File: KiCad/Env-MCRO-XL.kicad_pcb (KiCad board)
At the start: 2 copper layers, 47 parts, among them SW1 RotaryEncoder_Switch, SW2 RotaryEncoder_Switch, SW3 RotaryEncoder_Switch, U1 Pico

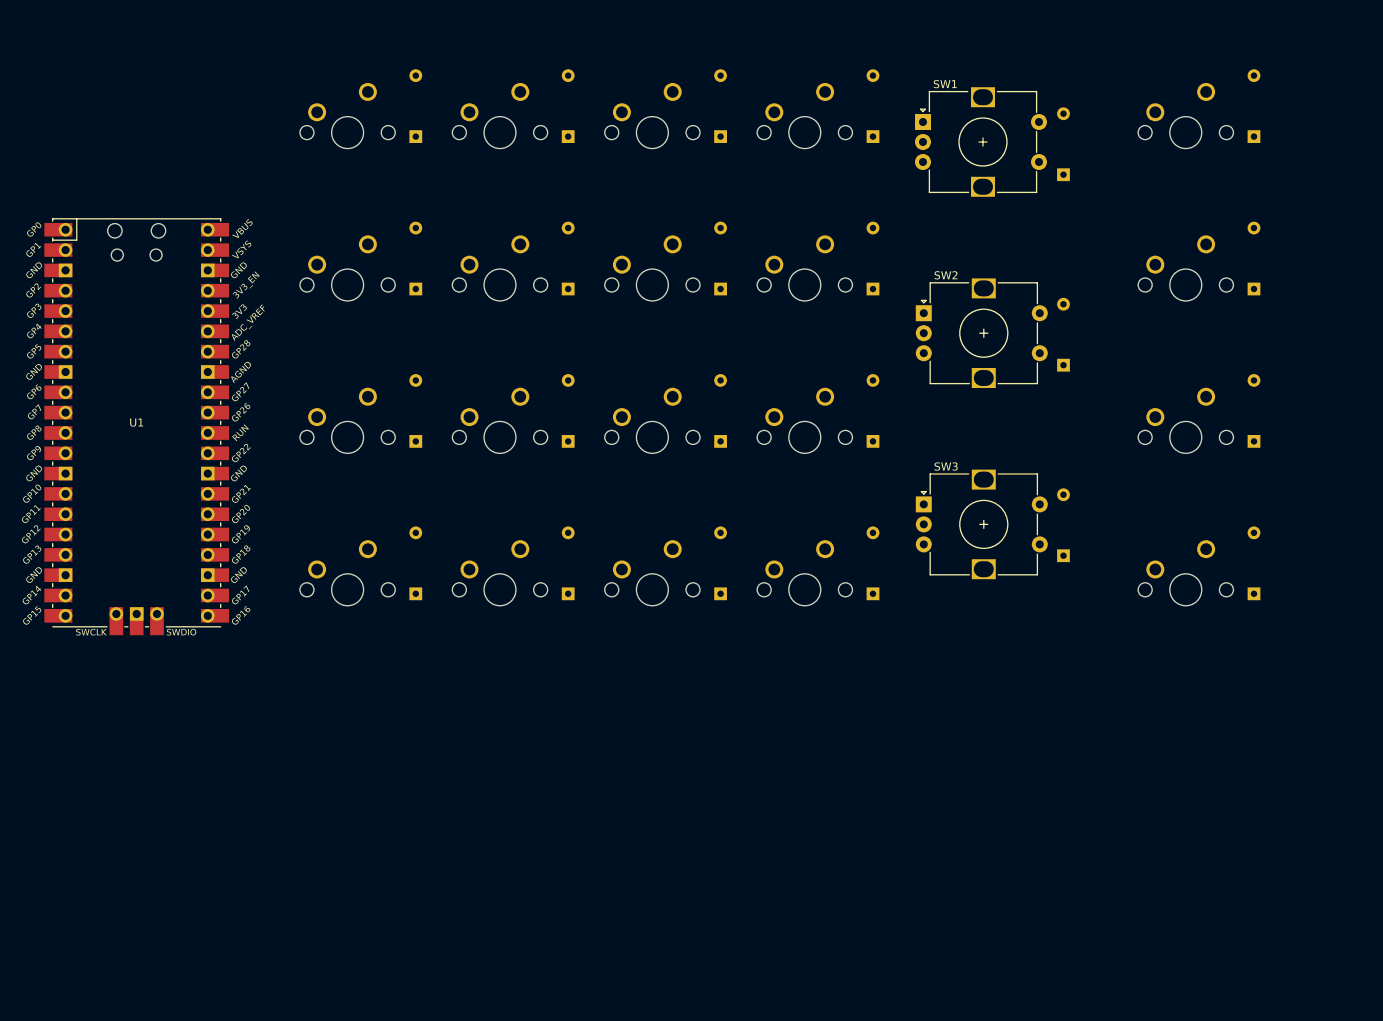
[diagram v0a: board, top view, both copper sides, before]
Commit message: initial commit + 2
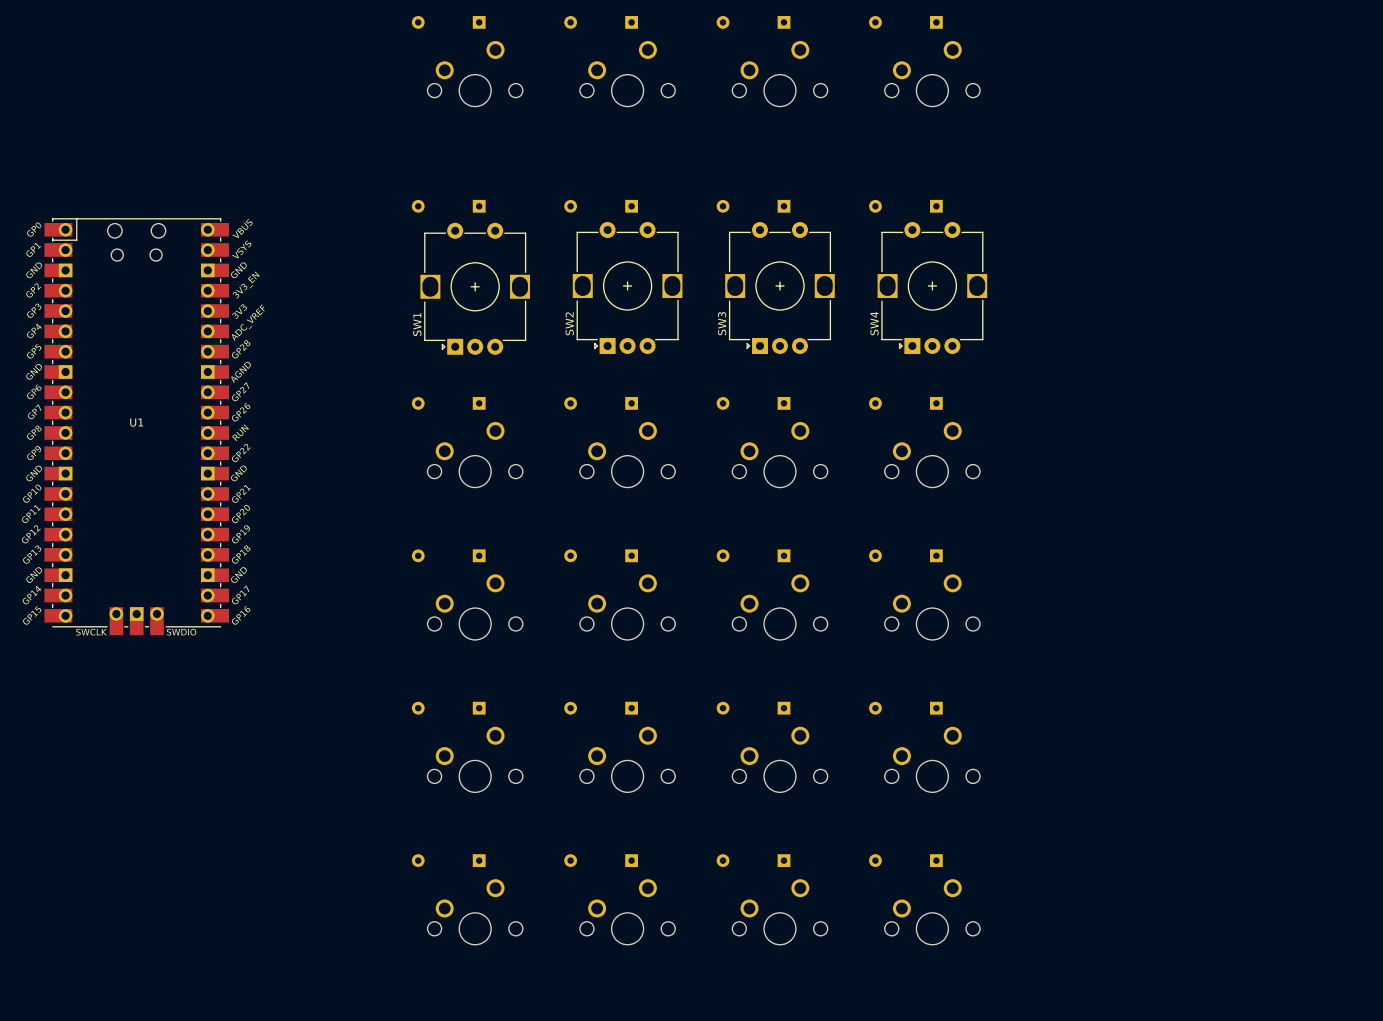
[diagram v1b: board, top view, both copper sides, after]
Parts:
- added D_21: 1n4148, Diode_THT:D_DO-35_SOD27_P7.62mm_Horizontal, B.Cu at (133.8, 48.3)
- added SW4: RotaryEncoder_Switch, Rotary_Encoder:RotaryEncoder_Alps_EC12E-Switch_Vertical_H20mm, F.Cu at (130.8, 65.8)
- moved K_0 100.8 mm to (76.2, 138.7)
- moved D_5 97.9 mm to (76.7, 25.4), turned to 180 degrees
- moved D_0 90.8 mm to (76.7, 130.1), turned to 180 degrees
- moved K_5 89.0 mm to (76.2, 33.9)
- moved K_6 87.8 mm to (95.2, 138.7)
- moved D_51 84.6 mm to (95.7, 25.4), turned to 180 degrees
- moved K_17 84.5 mm to (133.3, 138.7)
- moved K_11 81.8 mm to (114.2, 138.7)
- moved D_151 81.7 mm to (133.8, 25.4), turned to 180 degrees
- moved K_1 80.5 mm to (76.2, 119.6)
- moved D_15 78.7 mm to (114.8, 25.4), turned to 180 degrees
- moved D_6 76.4 mm to (95.7, 130.1), turned to 180 degrees
- moved K_51 73.9 mm to (95.2, 33.9)
- moved D_4 73.1 mm to (76.7, 48.3), turned to 180 degrees
- moved D_17 73.1 mm to (133.8, 130.1), turned to 180 degrees
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
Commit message: Settled on design and wired it up.
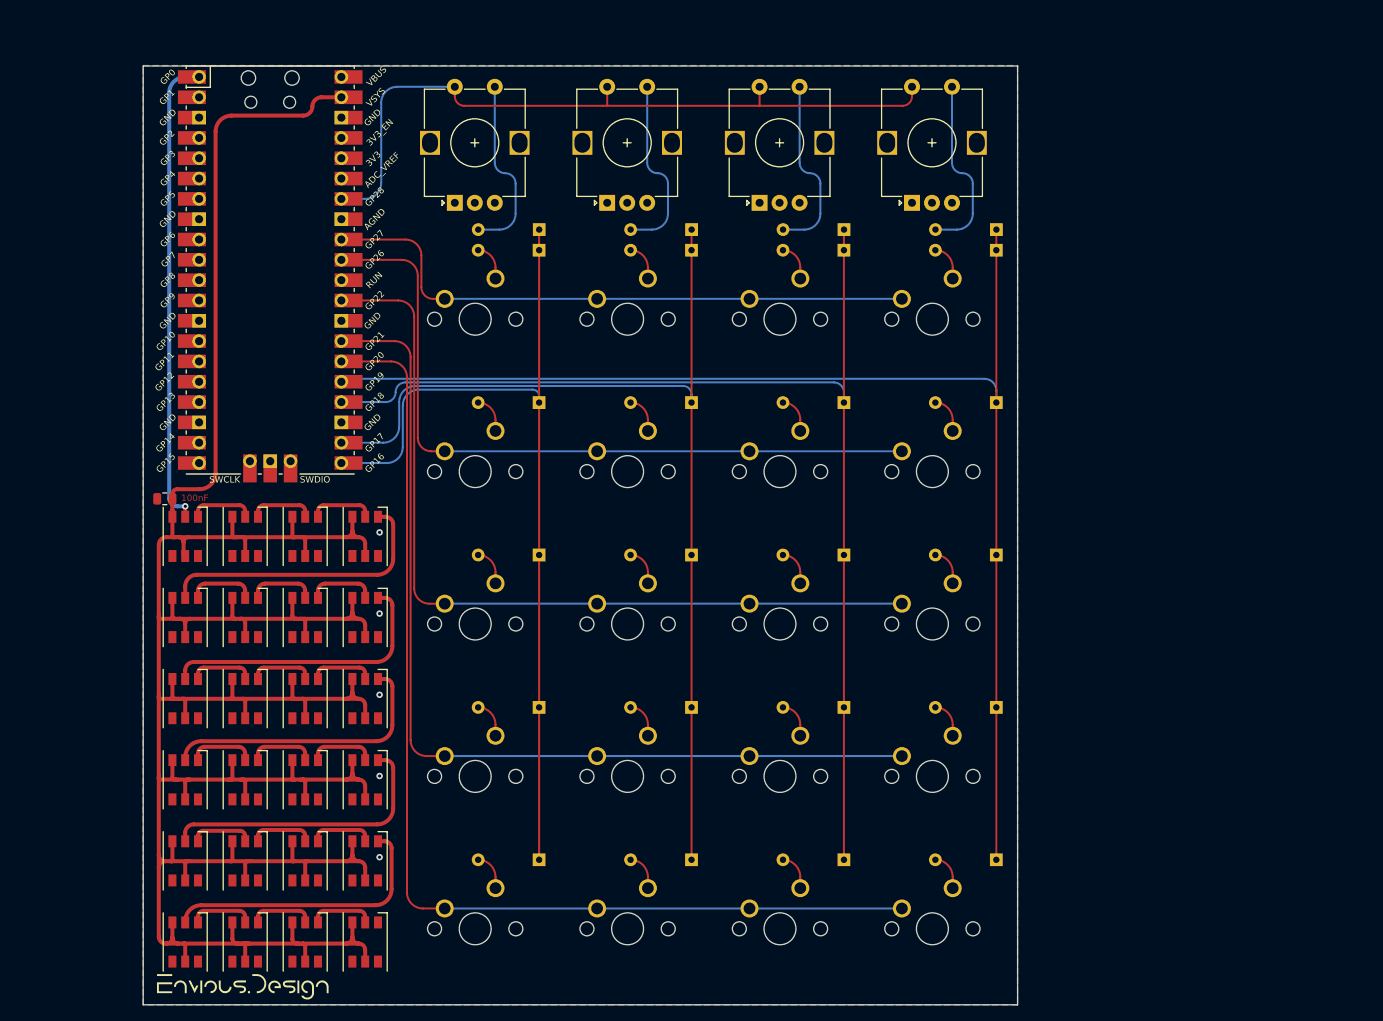
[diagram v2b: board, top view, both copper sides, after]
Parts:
- added C1: 100nf, Capacitor_SMD:C_0805_2012Metric, F.Cu at (37.4, 84.9)
- added RGB1: WS2812, LED_SMD:LED_WS2812_PLCC6_5.0x5.0mm_P1.6mm, F.Cu at (39.9, 89.6)
- added RGB10: WS2812, LED_SMD:LED_WS2812_PLCC6_5.0x5.0mm_P1.6mm, F.Cu at (47.4, 109.9)
- added RGB11: WS2812, LED_SMD:LED_WS2812_PLCC6_5.0x5.0mm_P1.6mm, F.Cu at (54.9, 109.9)
- added RGB12: WS2812, LED_SMD:LED_WS2812_PLCC6_5.0x5.0mm_P1.6mm, F.Cu at (62.4, 109.9)
- added RGB13: WS2812, LED_SMD:LED_WS2812_PLCC6_5.0x5.0mm_P1.6mm, F.Cu at (39.9, 120.0)
- added RGB14: WS2812, LED_SMD:LED_WS2812_PLCC6_5.0x5.0mm_P1.6mm, F.Cu at (47.4, 120.0)
- added RGB15: WS2812, LED_SMD:LED_WS2812_PLCC6_5.0x5.0mm_P1.6mm, F.Cu at (54.9, 120.0)
- added RGB16: WS2812, LED_SMD:LED_WS2812_PLCC6_5.0x5.0mm_P1.6mm, F.Cu at (62.4, 120.0)
- added RGB17: WS2812, LED_SMD:LED_WS2812_PLCC6_5.0x5.0mm_P1.6mm, F.Cu at (39.9, 130.2)
- added RGB18: WS2812, LED_SMD:LED_WS2812_PLCC6_5.0x5.0mm_P1.6mm, F.Cu at (47.4, 130.2)
- added RGB19: WS2812, LED_SMD:LED_WS2812_PLCC6_5.0x5.0mm_P1.6mm, F.Cu at (54.9, 130.2)
- added RGB2: WS2812, LED_SMD:LED_WS2812_PLCC6_5.0x5.0mm_P1.6mm, F.Cu at (47.4, 89.6)
- added RGB20: WS2812, LED_SMD:LED_WS2812_PLCC6_5.0x5.0mm_P1.6mm, F.Cu at (62.4, 130.2)
- added RGB21: WS2812, LED_SMD:LED_WS2812_PLCC6_5.0x5.0mm_P1.6mm, F.Cu at (39.9, 140.3)
- added RGB22: WS2812, LED_SMD:LED_WS2812_PLCC6_5.0x5.0mm_P1.6mm, F.Cu at (47.4, 140.3)
- added RGB23: WS2812, LED_SMD:LED_WS2812_PLCC6_5.0x5.0mm_P1.6mm, F.Cu at (54.9, 140.3)
- added RGB24: WS2812, LED_SMD:LED_WS2812_PLCC6_5.0x5.0mm_P1.6mm, F.Cu at (62.4, 140.3)
- added RGB3: WS2812, LED_SMD:LED_WS2812_PLCC6_5.0x5.0mm_P1.6mm, F.Cu at (54.9, 89.6)
- added RGB4: WS2812, LED_SMD:LED_WS2812_PLCC6_5.0x5.0mm_P1.6mm, F.Cu at (62.4, 89.6)
- added RGB5: WS2812, LED_SMD:LED_WS2812_PLCC6_5.0x5.0mm_P1.6mm, F.Cu at (39.9, 99.7)
- added RGB6: WS2812, LED_SMD:LED_WS2812_PLCC6_5.0x5.0mm_P1.6mm, F.Cu at (47.4, 99.7)
- added RGB7: WS2812, LED_SMD:LED_WS2812_PLCC6_5.0x5.0mm_P1.6mm, F.Cu at (54.9, 99.7)
- added RGB8: WS2812, LED_SMD:LED_WS2812_PLCC6_5.0x5.0mm_P1.6mm, F.Cu at (62.4, 99.7)
- added RGB9: WS2812, LED_SMD:LED_WS2812_PLCC6_5.0x5.0mm_P1.6mm, F.Cu at (39.9, 109.9)
- added kibuzzard-62A3132E: G***, kibuzzard-62A3132E, F.Cu at (47.1, 145.9)
- moved D_15 29.4 mm to (122.2, 53.8)
- moved D_151 29.4 mm to (141.3, 53.8)
- moved D_5 29.4 mm to (84.1, 53.8)
- moved D_51 29.4 mm to (103.2, 53.8)
- moved K_15 28.6 mm to (114.2, 62.5)
- moved K_151 28.6 mm to (133.3, 62.5)
- moved K_5 28.6 mm to (76.2, 62.5)
- moved K_51 28.6 mm to (95.2, 62.5)
- moved U1 25.4 mm to (50.5, 56.3)
- moved SW1 18.0 mm to (73.6, 47.9)
- moved SW2 17.9 mm to (92.7, 47.9)
- moved SW3 17.9 mm to (111.7, 47.9)
- moved SW4 17.9 mm to (130.8, 47.9)
- moved D_10 8.05 mm to (103.2, 51.2)
- moved D_16 8.05 mm to (122.3, 51.2)
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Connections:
- D_10 pad 2: ROT_SW2-A -> /SWROT2-B
- D_16 pad 2: ROT_SW3-A -> /SWROT3-B
- D_21 pad 2: ROT_SW4-A -> /SWROT4-B
- D_4 pad 2: ROT_SW1-A -> /SWROT1-B
- K_15 pad 1: col5 -> col4
- K_151 pad 1: col5 -> col4
- K_5 pad 1: col5 -> col4
- K_51 pad 1: col5 -> col4
- SW1 pad C: unconnected-(SW1-PadC) -> GND
- SW1 pad S1: ROT_SW1-A -> col5
- SW1 pad S2: ROT_SW1-B -> /SWROT1-B
- SW2 pad C: unconnected-(SW2-PadC) -> GND
- SW2 pad S1: ROT_SW2-A -> col5
- SW2 pad S2: ROT_SW1-B -> /SWROT2-B
- SW3 pad C: unconnected-(SW3-PadC) -> GND
- SW3 pad S1: ROT_SW3-A -> col5
- SW3 pad S2: ROT_SW1-B -> /SWROT3-B
- SW4 pad C: unconnected-(SW4-PadC) -> GND
- SW4 pad S1: ROT_SW4-A -> col5
- SW4 pad S2: ROT_SW1-B -> /SWROT4-B
- U1 pad 1: unconnected-(U1-Pad1) -> GP0
- U1 pad 13: unconnected-(U1-Pad13) -> GND
- U1 pad 18: unconnected-(U1-Pad18) -> GND
- U1 pad 21: unconnected-(U1-Pad21) -> row0
- U1 pad 22: unconnected-(U1-Pad22) -> row1
- U1 pad 23: unconnected-(U1-Pad23) -> GND
- U1 pad 24: unconnected-(U1-Pad24) -> row2
- U1 pad 25: unconnected-(U1-Pad25) -> row3
- U1 pad 26: unconnected-(U1-Pad26) -> col0
- U1 pad 27: unconnected-(U1-Pad27) -> col1
- U1 pad 28: unconnected-(U1-Pad28) -> GND
- U1 pad 29: unconnected-(U1-Pad29) -> col2
- U1 pad 3: unconnected-(U1-Pad3) -> GND
- U1 pad 31: unconnected-(U1-Pad31) -> col3
- U1 pad 32: unconnected-(U1-Pad32) -> col4
- U1 pad 33: unconnected-(U1-Pad33) -> GND
- U1 pad 34: unconnected-(U1-Pad34) -> col5
- U1 pad 38: unconnected-(U1-Pad38) -> GND
- U1 pad 39: unconnected-(U1-Pad39) -> +5V
- U1 pad 8: unconnected-(U1-Pad8) -> GND
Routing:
- net +5V: track 0.00 -> 409.0 mm
- net row3: track 0.00 -> 162.7 mm
- net row2: track 0.00 -> 144.8 mm
- net col0: track 0.00 -> 136.6 mm
- net row1: track 0.00 -> 129.3 mm
- net col1: track 0.00 -> 120.1 mm
- net row0: track 0.00 -> 112.0 mm
- net col2: track 0.00 -> 106.1 mm
- net col3: track 0.00 -> 92.3 mm
- net col5: track 0.00 -> 91.9 mm
- net col4: track 0.00 -> 75.9 mm
- net GP0: track 0.00 -> 59.3 mm, vias 0 -> 1
- net Net-(RGB16-Pad1): track 0.00 -> 36.2 mm
- net Net-(RGB8-Pad1): track 0.00 -> 36.0 mm
- net Net-(RGB4-Pad1): track 0.00 -> 36.0 mm
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- added copper zone on B.Cu, net GND
- added copper zone on F.Cu, net GND
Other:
- board outline added: 109.3 x 117.4 mm
- board text added: "100nF"

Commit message: various changes and all that.
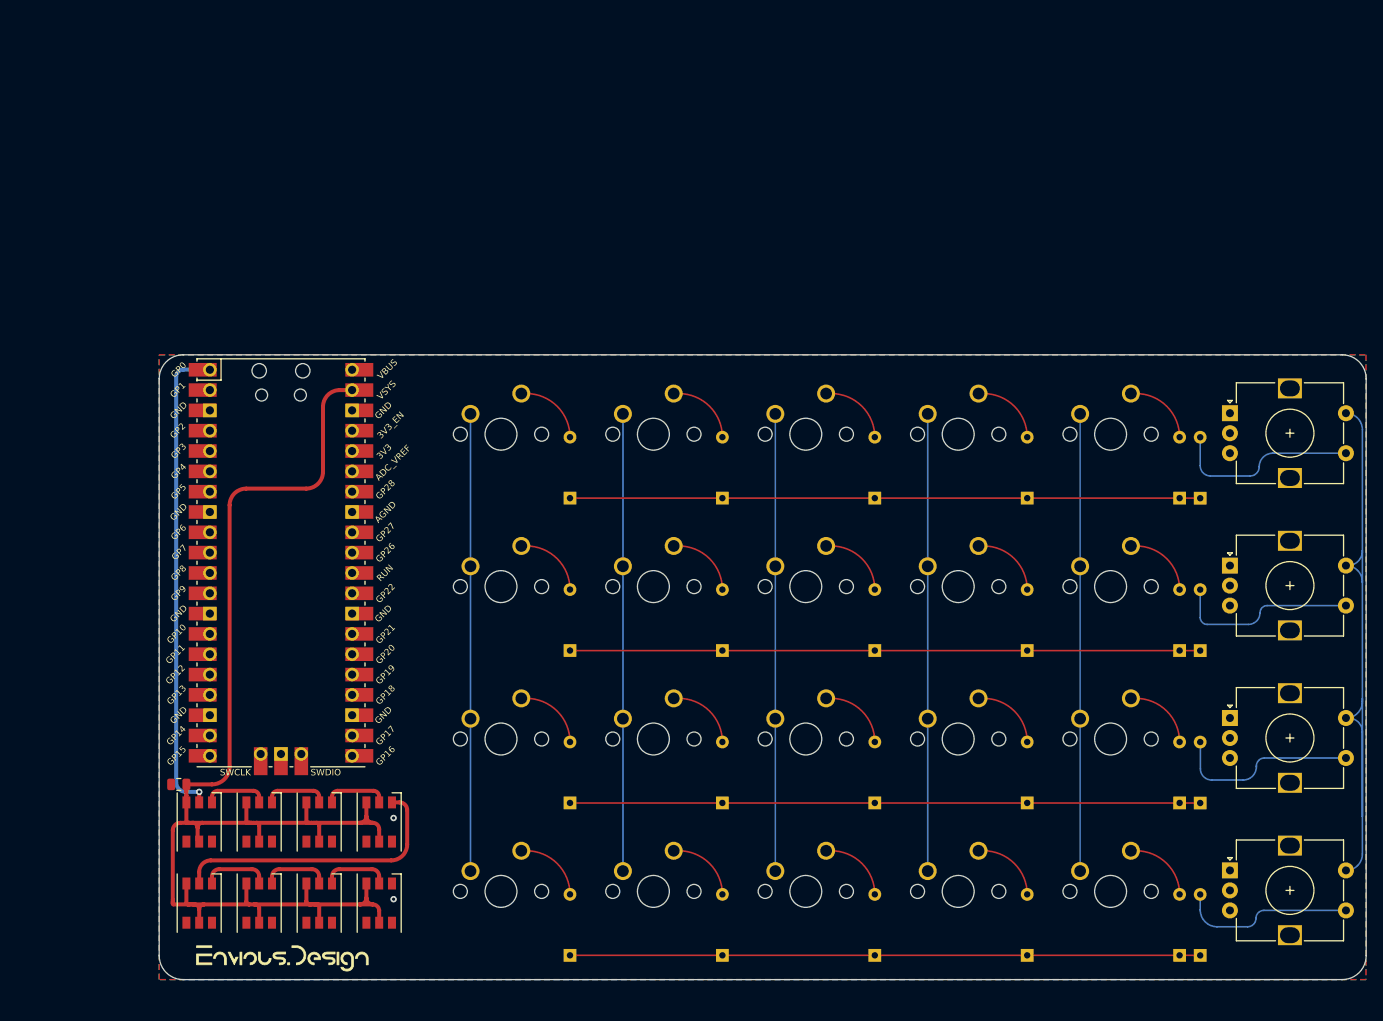
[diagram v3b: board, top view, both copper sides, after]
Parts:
- removed RGB10, RGB11, RGB12, RGB13, RGB14, RGB15, RGB16, RGB17, RGB18, RGB19, RGB20, RGB21, RGB22, RGB23, RGB24, RGB9: WS2812, LED_SMD:LED_WS2812_PLCC6_5.0x5.0mm_P1.6mm
- moved SW1 100.4 mm to (170.5, 74.2), turned to 0 degrees
- moved D_21 94.2 mm to (166.8, 142.0), turned to 90 degrees
- moved SW4 92.4 mm to (170.5, 131.3), turned to 0 degrees
- moved D_151 91.1 mm to (164.2, 142.0), turned to 90 degrees
- moved SW2 90.1 mm to (170.5, 93.2), turned to 0 degrees
- moved D_4 89.2 mm to (166.8, 84.8), turned to 90 degrees
- moved SW3 87.2 mm to (170.5, 112.3), turned to 0 degrees
- moved D_5 85.8 mm to (164.2, 84.8), turned to 90 degrees
- moved D_16 84.4 mm to (166.8, 122.9), turned to 90 degrees
- moved D_10 82.5 mm to (166.8, 103.9), turned to 90 degrees
- moved D_15 80.8 mm to (164.2, 122.9), turned to 90 degrees
- moved K_5 80.7 mm to (155.6, 76.8)
- moved D_51 78.9 mm to (164.2, 103.9), turned to 90 degrees
- moved K_151 74.9 mm to (155.6, 134.0)
- moved D_20 69.2 mm to (145.2, 142.0), turned to 90 degrees
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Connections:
- U1 pad 21: row0 -> unconnected-(U1-Pad21)
- U1 pad 22: row1 -> unconnected-(U1-Pad22)
- U1 pad 24: row2 -> unconnected-(U1-Pad24)
- U1 pad 25: row3 -> unconnected-(U1-Pad25)
- U1 pad 26: col0 -> unconnected-(U1-Pad26)
- U1 pad 27: col1 -> unconnected-(U1-Pad27)
- U1 pad 29: col2 -> unconnected-(U1-Pad29)
- U1 pad 31: col3 -> unconnected-(U1-Pad31)
- U1 pad 32: col4 -> unconnected-(U1-Pad32)
- U1 pad 34: col5 -> unconnected-(U1-Pad34)
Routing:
- net +5V: track 409.0 -> 173.9 mm
- net row3: track 162.7 -> 78.8 mm
- net col0: track 136.6 -> 57.2 mm
- net row2: track 144.8 -> 78.8 mm
- net col1: track 120.1 -> 57.2 mm
- net row1: track 129.3 -> 78.8 mm
- net col2: track 106.1 -> 57.2 mm
- net Net-(RGB16-Pad1): track 36.2 -> 0.00 mm
- net Net-(RGB8-Pad1): track 36.0 -> 0.00 mm
- net Net-(RGB20-Pad1): track 35.2 -> 0.00 mm
- net Net-(RGB12-Pad1): track 35.2 -> 0.00 mm
- net col3: track 92.3 -> 57.2 mm
- net row0: track 112.0 -> 78.8 mm
- net col4: track 75.9 -> 57.2 mm
- net col5: track 91.9 -> 82.5 mm
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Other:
- board size 109.3 x 117.4 mm -> 150.9 x 78.1 mm
- board text removed: "100nF"

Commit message: decided to revamp this project a tad.
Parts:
- removed C1: 100nf, Capacitor_SMD:C_0805_2012Metric
- removed D_0, D_1, D_10, D_11, D_12, D_13, D_14, D_15, D_151, D_16, D_17, D_18, D_19, D_2, D_20, D_21, D_3, D_4, D_5, D_51, D_6, D_7, D_8, D_9: 1n4148, Diode_THT:D_DO-35_SOD27_P7.62mm_Horizontal
- removed K_0, K_1, K_11, K_12, K_13, K_14, K_15, K_151, K_17, K_18, K_19, K_2, K_20, K_3, K_5, K_51, K_6, K_7, K_8, K_9: MX Switch, MX_Only:MXOnly-1U-NoLED
- removed RGB1, RGB2, RGB3, RGB4, RGB5, RGB6, RGB7, RGB8: WS2812, LED_SMD:LED_WS2812_PLCC6_5.0x5.0mm_P1.6mm
- removed SW1, SW2, SW3, SW4: RotaryEncoder_Switch, Rotary_Encoder:RotaryEncoder_Alps_EC12E-Switch_Vertical_H20mm
- removed U1: Pico, MCU_RaspberryPi_and_Boards:RPi_Pico_SMD_TH
- removed kibuzzard-62A3132E: G***, kibuzzard-62A3132E
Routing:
- net +5V: track 173.9 -> 0.00 mm
- net col5: track 82.5 -> 0.00 mm
- net row1: track 78.8 -> 0.00 mm
- net row2: track 78.8 -> 0.00 mm
- net row3: track 78.8 -> 0.00 mm
- net row0: track 78.8 -> 0.00 mm
- net GP0: track 60.2 -> 0.00 mm, vias 1 -> 0
- net col4: track 57.2 -> 0.00 mm
- net col3: track 57.2 -> 0.00 mm
- net col2: track 57.2 -> 0.00 mm
- net col1: track 57.2 -> 0.00 mm
- net col0: track 57.2 -> 0.00 mm
- net Net-(RGB4-Pad1): track 36.0 -> 0.00 mm
- net /SWROT1-B: track 24.0 -> 0.00 mm
- net /SWROT3-B: track 23.8 -> 0.00 mm
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- removed copper zone on B.Cu, net GND
- removed copper zone on F.Cu, net GND
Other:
- board outline removed
